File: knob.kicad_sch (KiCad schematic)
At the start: 8 parts, among them J1 SJ2-35464B-SMT-TR

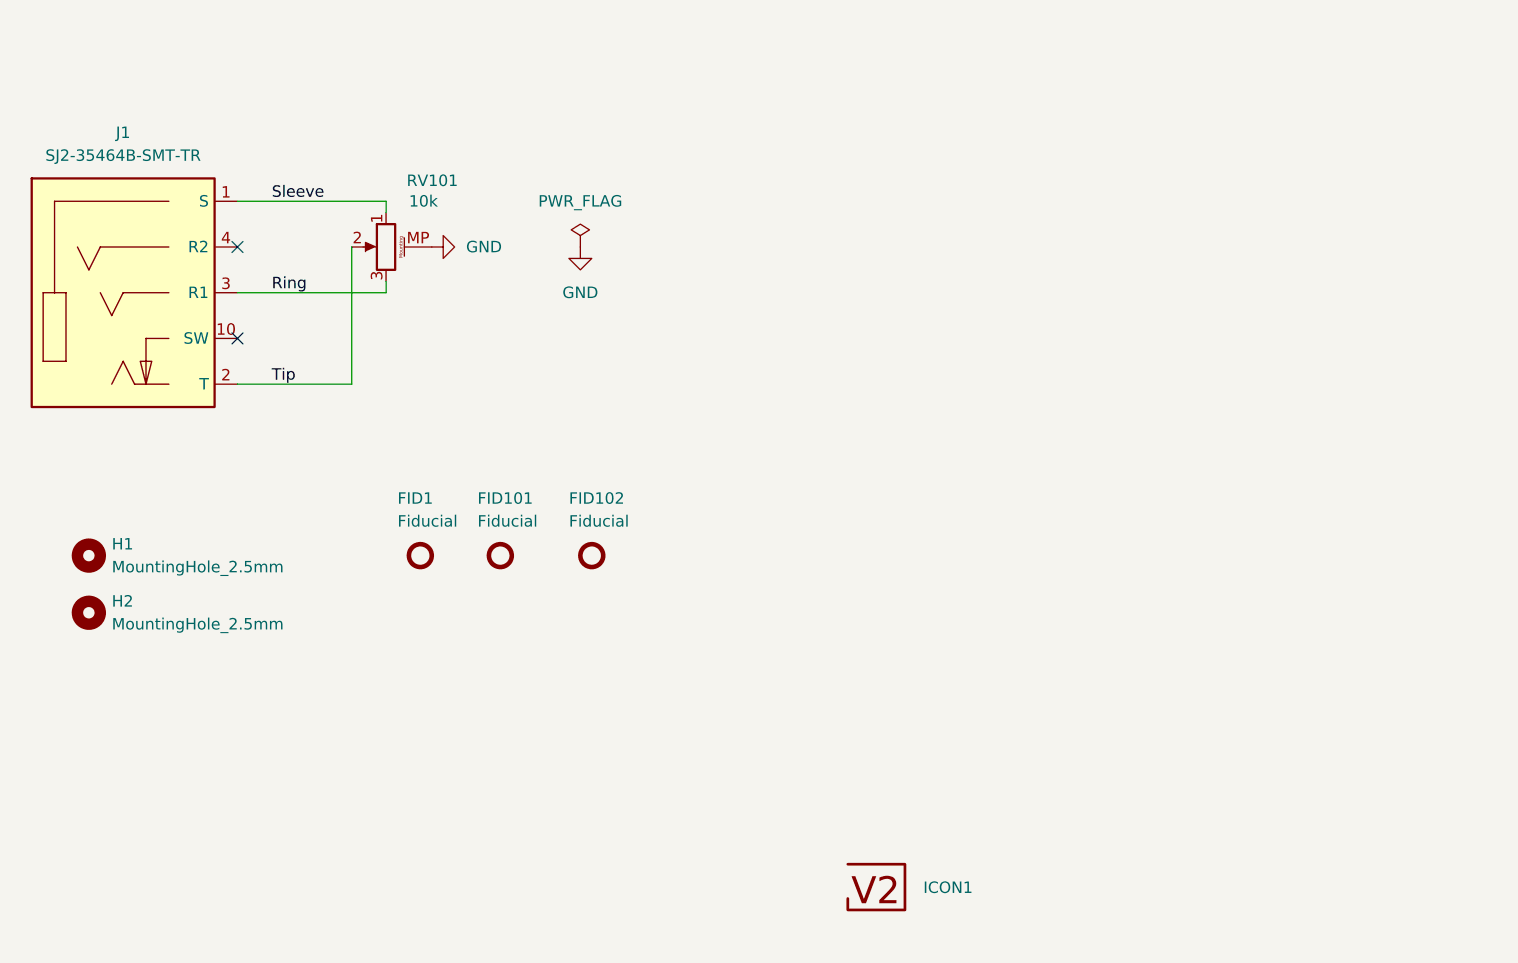
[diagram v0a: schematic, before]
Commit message: Update Library
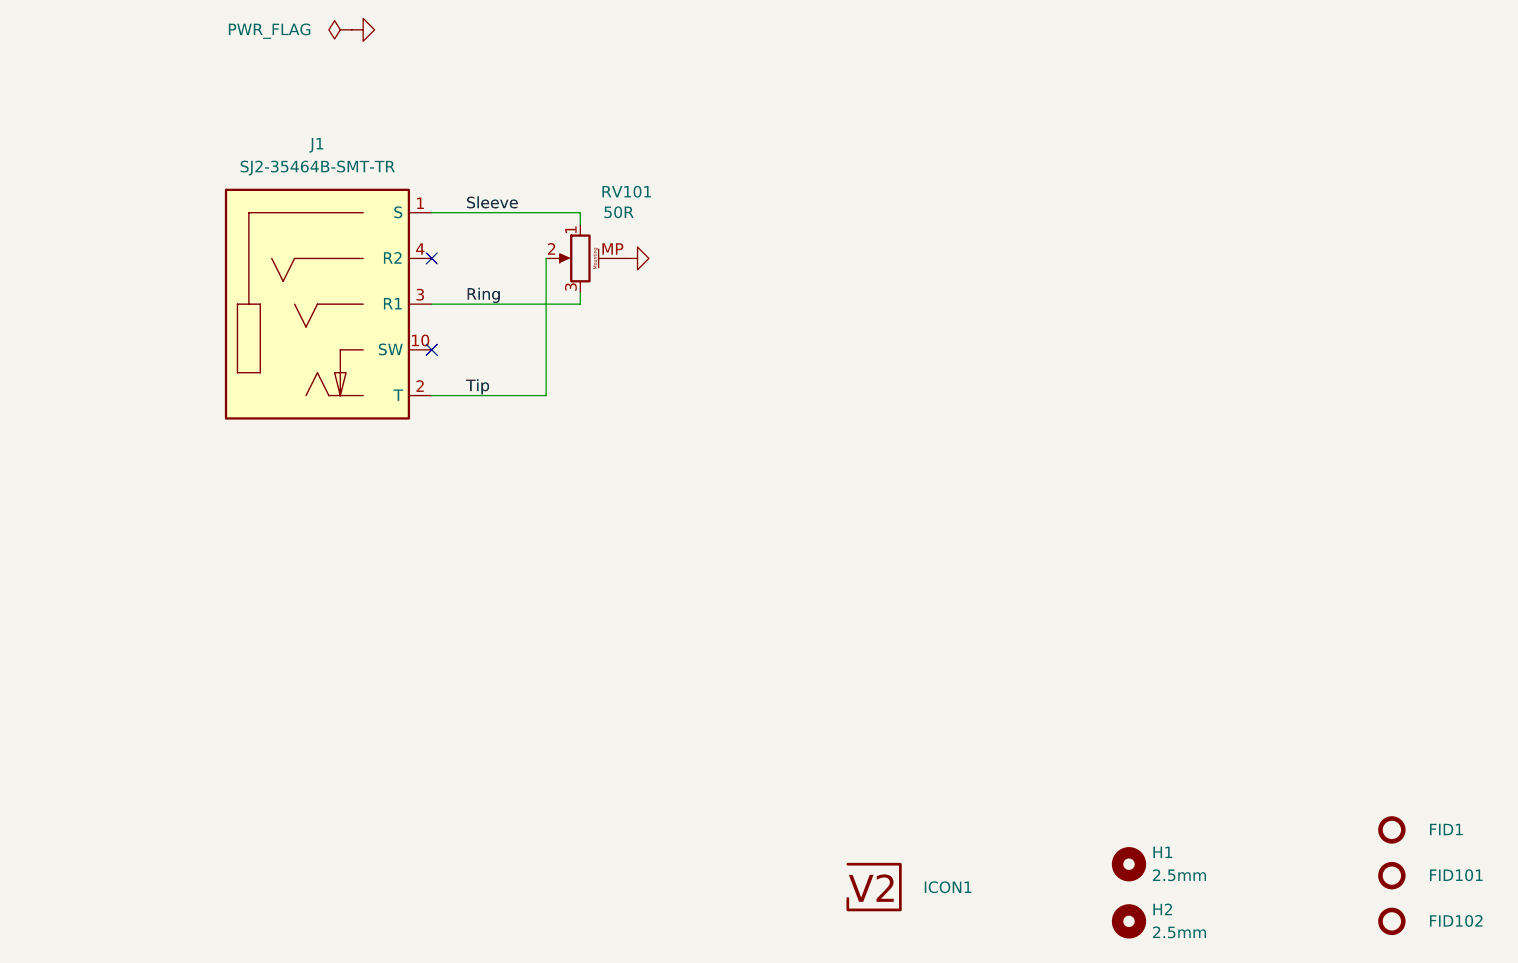
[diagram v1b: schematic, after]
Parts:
- FID1, FID101, FID102: value Fiducial -> Fiducial_Paste
- H1, H2: value MountingHole_2.5mm -> 2.5mm
- J1: Manufacturer (none) -> Same Sky; Mouser (none) -> 490-SJ2-35464BSMT-TR; Product (none) -> SJ2-35464B-SMT-TR
- RV101: value 10k -> 50R; symbol Device:R_Potentiometer_MountingPin -> V2_Potentiometer:MountingPin_50R
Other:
- moved on the sheet: FID1, FID101, FID102, H1, H2, J1, RV101
